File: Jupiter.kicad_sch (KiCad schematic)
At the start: 341 parts, among them J1 Conn_01x04, SW1 SW_Push, U1 ATmega32U4-M, Y1 Crystal_GND24_Small

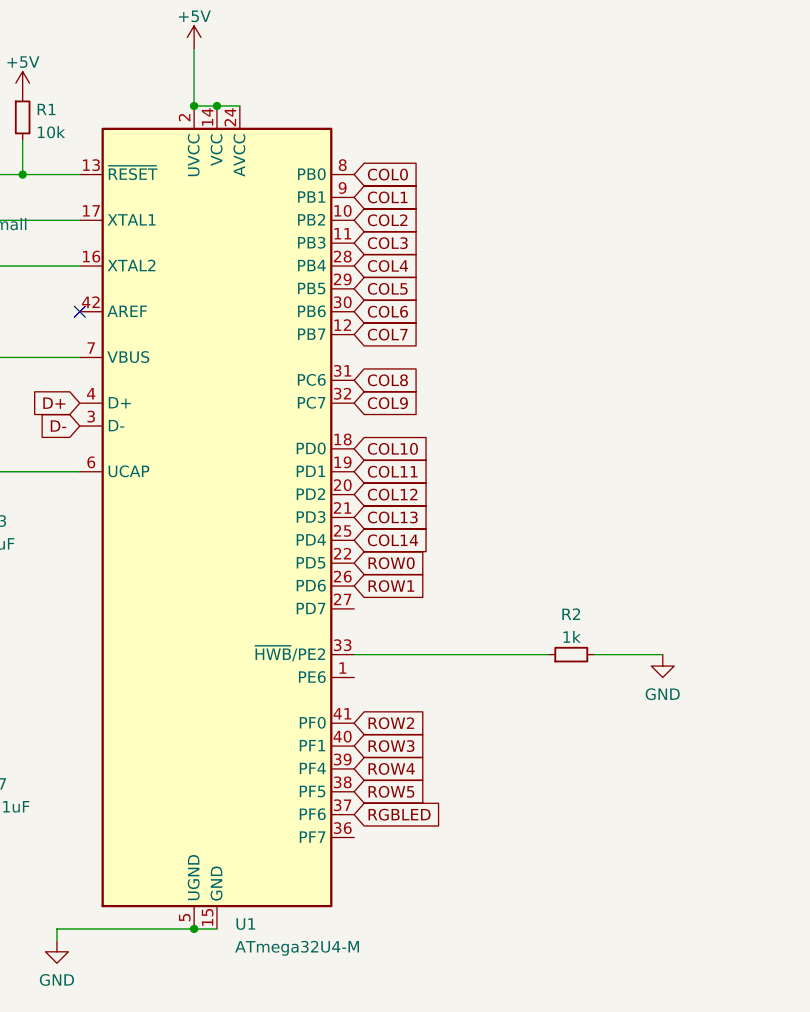
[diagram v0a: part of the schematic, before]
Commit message: traces
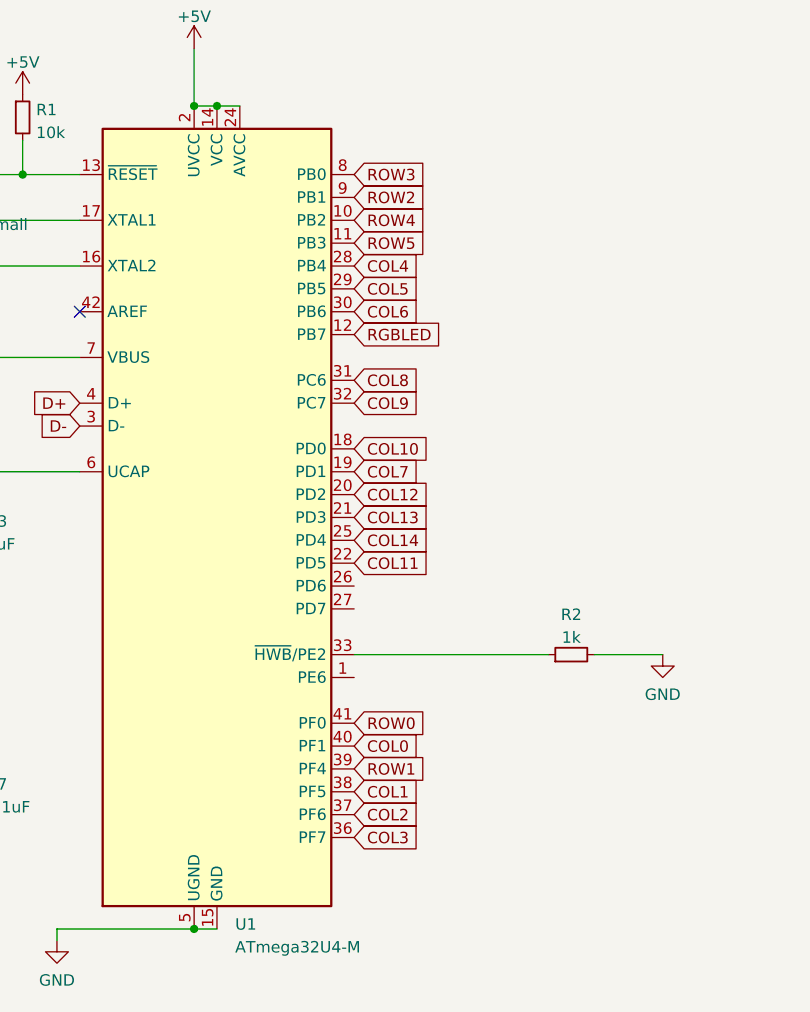
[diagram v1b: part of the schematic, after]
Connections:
- net COL0: now also U1.40 (PF1); no longer U1.8 (PB0)
- net COL1: now also U1.38 (PF5); no longer U1.9 (PB1)
- net COL11: now also U1.22 (PD5); no longer U1.19 (PD1)
- net COL2: now also U1.37 (PF6); no longer U1.10 (PB2)
- net COL3: now also U1.36 (PF7); no longer U1.11 (PB3)
- net COL7: now also U1.19 (PD1); no longer U1.12 (PB7)
- net RGBLED: now also U1.12 (PB7); no longer U1.37 (PF6)
- net ROW0: now also U1.41 (PF0); no longer U1.22 (PD5)
- net ROW1: now also U1.39 (PF4); no longer U1.26 (PD6)
- net ROW2: now also U1.9 (PB1); no longer U1.41 (PF0)
- net ROW3: now also U1.8 (PB0); no longer U1.40 (PF1)
- net ROW4: now also U1.10 (PB2); no longer U1.39 (PF4)
- net ROW5: now also U1.11 (PB3); no longer U1.38 (PF5)

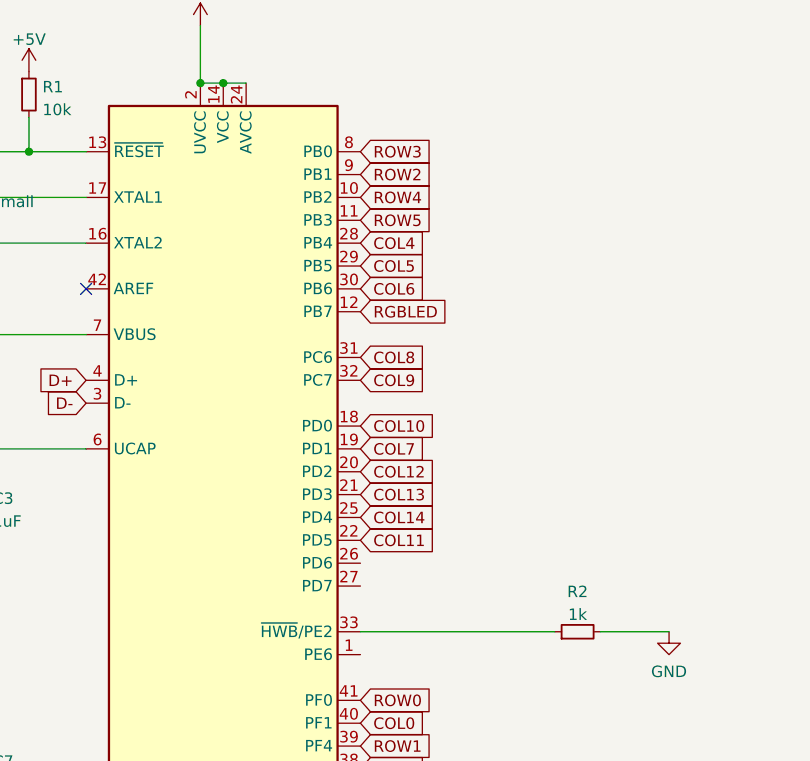
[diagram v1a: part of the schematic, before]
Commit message: more traces
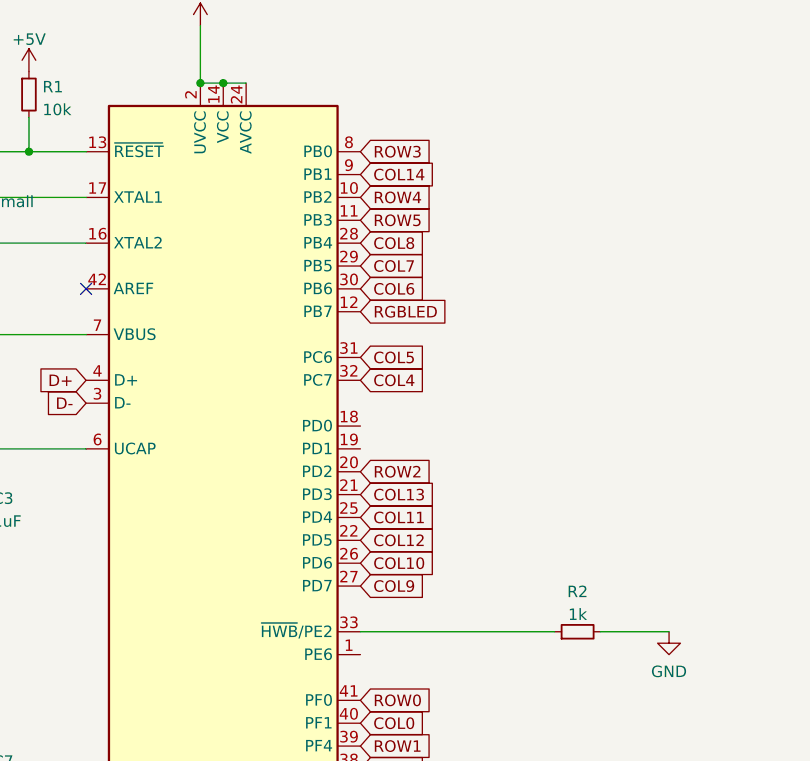
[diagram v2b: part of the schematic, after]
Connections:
- net COL10: now also U1.26 (PD6); no longer U1.18 (PD0)
- net COL11: now also U1.25 (PD4); no longer U1.22 (PD5)
- net COL12: now also U1.22 (PD5); no longer U1.20 (PD2)
- net COL14: now also U1.9 (PB1); no longer U1.25 (PD4)
- net COL4: now also U1.32 (PC7); no longer U1.28 (PB4)
- net COL5: now also U1.31 (PC6); no longer U1.29 (PB5)
- net COL7: now also U1.29 (PB5); no longer U1.19 (PD1)
- net COL8: now also U1.28 (PB4); no longer U1.31 (PC6)
- net COL9: now also U1.27 (PD7); no longer U1.32 (PC7)
- net ROW2: now also U1.20 (PD2); no longer U1.9 (PB1)

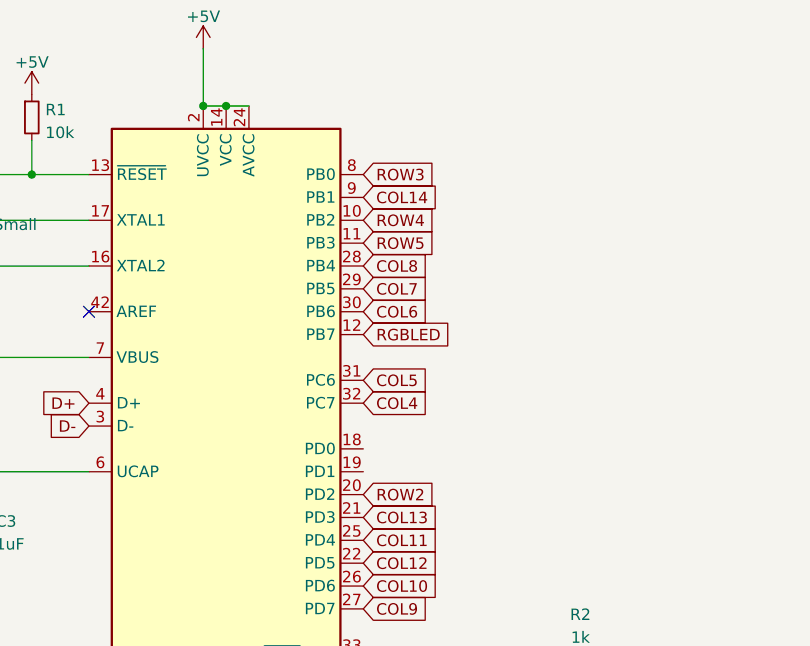
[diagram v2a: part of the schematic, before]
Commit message: almost finished trace routing
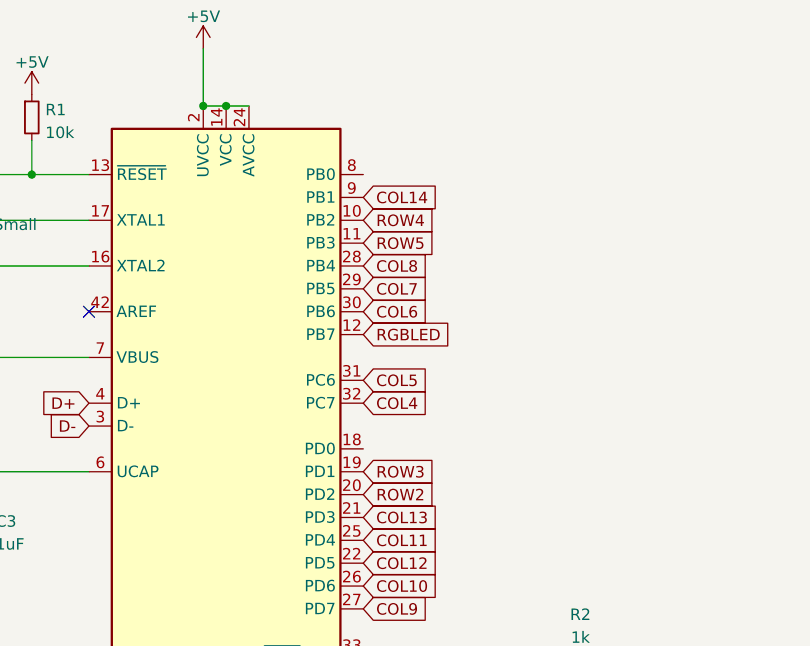
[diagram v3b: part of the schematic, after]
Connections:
- net ROW3: now also U1.19 (PD1); no longer U1.8 (PB0)
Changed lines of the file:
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@@
+    )
+  )
+  (global_label "ROW3" (shape input) (at 391.16 67.31 0) (fields_autoplaced)
+    (effects (font (size 1.27 1.27)) (justify left))
+    (property "Intersheet References" "${INTERSHEET_REFS}" (id 0) (at 398.8345 67.3894 0)
+      (effects (font (size 1.27 1.27)) (justify left) hide)
     )
   )
@@
       (effects (font (size 1.27 1.27)) (justify left) hide)
     )
-  )
-  (global_label "ROW3" (shape input) (at 391.16 34.29 0) (fields_autoplaced)
-    (effects (font (size 1.27 1.27)) (justify left))
-    (property "Intersheet References" "${INTERSHEET_REFS}" (id 0) (at 398.8345 34.3694 0)
-      (effects (font (size 1.27 1.27)) (justify left) hide)
-    )
